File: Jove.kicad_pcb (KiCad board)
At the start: 2 copper layers, 65 x 100 mm, 156 parts, among them J1 PJ301B, J2 PJ301B, J3 PJ301B, J4 PJ301B, J5 PJ301B, J6 PJ301B, P1 CONN_02X05, Q1 BCM857BS, Q2 BCM857BS, Q3 J112, Q4 J112, Q5 J112, Q6 J112, SW1 KS-01Q, U1 TL072-, U10 CD4027, U11 CD40106, U12 TS321, U13 TS321, U2 TL072-, U3 TL072-, U4 TL072-, U5 LM13700, U6 LM13700, U7 LM13700, U8 DG409, U9 CD4052

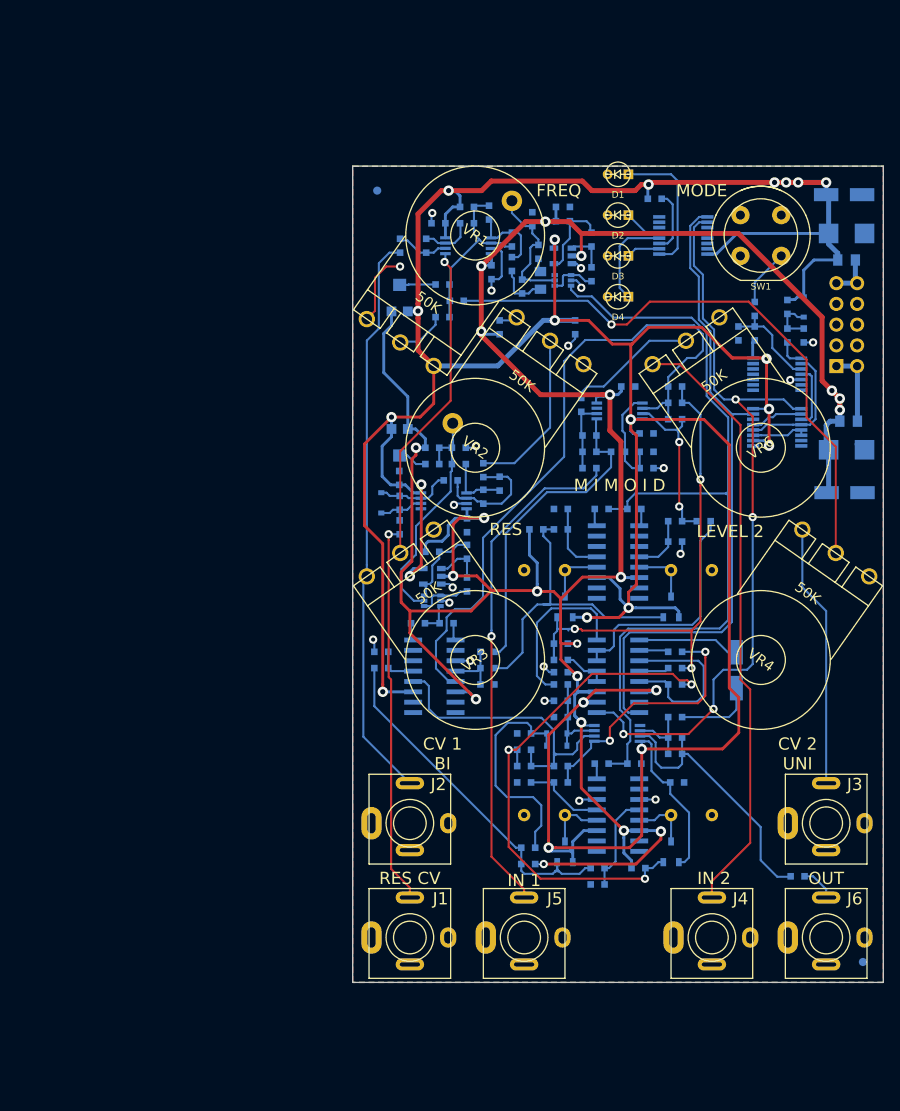
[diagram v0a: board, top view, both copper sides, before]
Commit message: redesign PCB
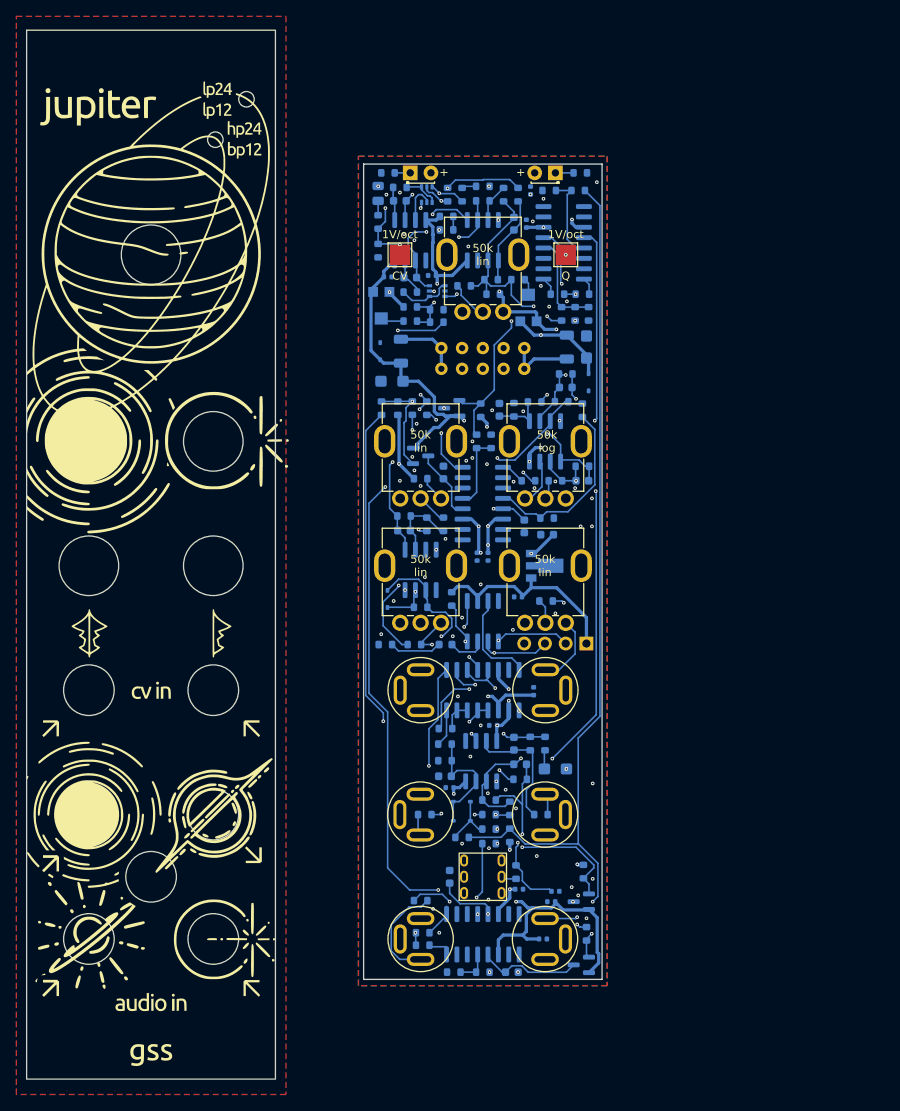
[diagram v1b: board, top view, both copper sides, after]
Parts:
- removed D4: LED, MyModules:3MM-LED-C1A2
- removed D7: 1N914, MyModules:SOD323-C1A2
- removed the REF** at (15.0, 15.0)
- removed the REF** at (74.5, 109.5)
- removed REF***: OSHW-Symbol_6.7x6mm_SilkScreen, Symbols:OSHW-Symbol_6.7x6mm_SilkScreen
- removed U11: CD40106, Housings_SSOP:TSSOP-14_4.4x5mm_Pitch0.65mm
- removed U13: TS321, TO_SOT_Packages_SMD:SOT-23-5
- added C30: 100n, Capacitor_SMD:C_0402_1005Metric, B.Cu at (36.8, 100.8)
- added C31: 100n, Capacitor_SMD:C_0402_1005Metric, B.Cu at (35.3, 106.7)
- added C32: 100n, Capacitor_SMD:C_0402_1005Metric, B.Cu at (32.4, 100.6)
- added G***: LOGO, LOGO, F.Cu at (-10.2, 59.4)
- added G***: LOGO, LOGO, F.Cu at (27.9, 59.4)
- added G***: LOGO, LOGO, F.Cu at (-12.8, 59.5)
- added J7: prog, Connector_PinHeader_2.54mm:PinHeader_1x04_P2.54mm_Vertical, B.Cu at (40.6, 70.5)
- added R79: 470k, Resistor_SMD:R_0603_1608Metric, B.Cu at (23.5, 18.2)
- added R80: 470k, Resistor_SMD:R_0603_1608Metric, B.Cu at (27.9, 14.5)
- added REF**: RK097_Drill_Hole_Panel, Genson_Drill_Holes:RK097_Drill_Hole_Panel, F.Cu at (-20.3, 45.7)
- added REF**: PJ392_Drill_Hole_Panel, Genson_Drill_Holes:PJ392_Drill_Hole_Panel, F.Cu at (-20.3, 76.2)
- added REF**: PJ392_Drill_Hole_Panel, Genson_Drill_Holes:PJ392_Drill_Hole_Panel, F.Cu at (-5.08, 91.4)
- added REF**: PJ392_Drill_Hole_Panel, Genson_Drill_Holes:PJ392_Drill_Hole_Panel, F.Cu at (-20.3, 91.4)
- added REF**: PJ392_Drill_Hole_Panel, Genson_Drill_Holes:PJ392_Drill_Hole_Panel, F.Cu at (-5.08, 76.2)
- added REF**: RK097_Drill_Hole_Panel, Genson_Drill_Holes:RK097_Drill_Hole_Panel, F.Cu at (-20.3, 61.0)
- added REF**: PJ392_Drill_Hole_Panel, Genson_Drill_Holes:PJ392_Drill_Hole_Panel, F.Cu at (-5.08, 106.7)
- added REF**: 6mm_cap_Drill_Hole_Panel, Genson_Drill_Holes:6mm_cap_Drill_Hole_Panel, F.Cu at (-12.7, 99.1)
- added REF**: PJ392_Drill_Hole_Panel, Genson_Drill_Holes:PJ392_Drill_Hole_Panel, F.Cu at (-20.3, 106.7)
- added REF**: LED_1.8mm_Drill_Hole_Panel, Genson_Drill_Holes:LED_1.8mm_Drill_Hole_Panel, F.Cu at (-4.83, 8.76)
- added REF**: RK097_Drill_Hole_Panel, Genson_Drill_Holes:RK097_Drill_Hole_Panel, F.Cu at (-12.7, 22.9)
- added REF**: 6HP_Front_Panel, Genson_Front_Panels:6HP_Front_Panel, F.Cu at (-27.9, -4.65)
- added REF**: RK097_Drill_Hole_Panel, Genson_Drill_Holes:RK097_Drill_Hole_Panel, F.Cu at (-5.08, 45.7)
- added REF**: LED_1.8mm_Drill_Hole_Panel, Genson_Drill_Holes:LED_1.8mm_Drill_Hole_Panel, F.Cu at (-1.02, 3.81)
- added REF**: RK097_Drill_Hole_Panel, Genson_Drill_Holes:RK097_Drill_Hole_Panel, F.Cu at (-5.08, 61.0)
- C1, C11, C2, C28, C29, C3, C4, C5, C8, C9: footprint MyModules:SM0603-C-JRL -> Capacitor_SMD:C_0603_1608Metric
- C10, C23, C24: footprint Capacitors_SMD:c_elec_5x5.3 -> Capacitor_Tantalum_SMD:CP_EIA-3216-18_Kemet-A
- C12, C13, C14, C15, C16, C17, C19, C20, C26, C27: footprint MyModules:SM0603-C-JRL -> Capacitor_SMD:C_0402_1005Metric
- C18, C25, C6, C7: footprint MyModules:CAP-BOX-PFR-5MM -> Capacitor_SMD:C_0603_1608Metric
- C21: value 0.47μ -> 330n; footprint MyModules:SM0603-C-JRL -> Capacitor_SMD:C_0603_1608Metric
- C22: value 0.47μ -> 100n; footprint MyModules:SM0603-C-JRL -> Capacitor_SMD:C_0402_1005Metric
- D1, D2: value LED -> red; footprint MyModules:3MM-LED-C1A2 -> LED_THT:LED_D1.8mm_W3.3mm_H2.4mm
- D10, D5, D6: footprint MyModules:SOD323-C1A2 -> Diode_SMD:D_SOD-323
- D3: value LED -> debug led; footprint MyModules:3MM-LED-C1A2 -> Diode_SMD:D_0603_1608Metric; moved to B.Cu
- D8, D9: value S1BB -> B5819WS; footprint MyModules:SMB-1C2A -> Diode_SMD:D_SOD-323
- J1: value PJ301B -> Resonance CV; footprint MyModules:PJ-301B-JACK-SLOTS -> Genson_Jacks:Jack_3.5mm_PJ392_Vertical
- J2: value PJ301B -> Bipolar Freq CV; footprint MyModules:PJ-301B-JACK-SLOTS -> Genson_Jacks:Jack_3.5mm_PJ392_Vertical
- J3: value PJ301B -> Unipolar Freq CV; footprint MyModules:PJ-301B-JACK-SLOTS -> Genson_Jacks:Jack_3.5mm_PJ392_Vertical
- J4, J5: value PJ301B -> Input2; footprint MyModules:PJ-301B-JACK-SLOTS -> Genson_Jacks:Jack_3.5mm_PJ392_Vertical
- J6: value PJ301B -> out; footprint MyModules:PJ-301B-JACK-SLOTS -> Genson_Jacks:Jack_3.5mm_PJ392_Vertical
- P1: footprint Pin_Headers:Pin_Header_Straight_2x05 -> Genson_Connectors:Eurorack_10Pin
- Q1, Q2: footprint SMD TRAN:sot323-6 -> Package_TO_SOT_SMD:SOT-363_SC-70-6
- Q3, Q4, Q5, Q6: footprint MyModules:SOT23-JRL -> Package_TO_SOT_SMD:SOT-23
- R1, R10, R11, R12, R13, R14, R15, R16, R17, R18, R2, R20, R22, R23, R24, R25, R26, R27, R29, R3, R30, R31, R32, R33, R34, R35, R36, R37, R38, R39, R4, R40, R42, R43, R44, R45, R46, R47, R48, R49, R5, R50, R51, R52, R53, R54, R55, R56, R57, R59, R6, R60, R62, R63, R64, R65, R68, R69, R7, R70, R71, R72, R73, R74, R75, R76, R77, R78, R8, R9: footprint MyModules:SM0603-R-JRL -> Resistor_SMD:R_0603_1608Metric
- R19: footprint MyModules:SM0805-HAND -> Resistor_SMD:R_0805_2012Metric
- R21, R28: value 1.5M -> 1M; footprint MyModules:SM0603-R-JRL -> Resistor_SMD:R_0603_1608Metric
- R41: value 3.3K -> 100k; footprint MyModules:SM0603-R-JRL -> Resistor_SMD:R_0603_1608Metric
- R58: value 33K -> 1k; footprint MyModules:SM0603-R-JRL -> Resistor_SMD:R_0603_1608Metric
- R61: value 100K -> 330; footprint MyModules:SM0603-R-JRL -> Resistor_SMD:R_0603_1608Metric
- R66, R67: footprint MyModules:SM0805-HAND -> Resistor_SMD:R_1206_3216Metric
- SW1: value KS-01Q -> SW_Push_DPDT; footprint synth:KS-01Q-02-JRL -> Genson_Switches:SW_5.8x5.8mm
- TP1, TP2: footprint MyModules:TEST POINT -> TestPoint:TestPoint_Pad_2.5x2.5mm; moved to F.Cu
- U1, U2, U3, U4: footprint MyModules:TSSOP8-JRL -> Package_SO:SOIC-8_3.9x4.9mm_P1.27mm
- U10: value CD4027 -> ~; footprint Housings_SSOP:TSSOP-16_4.4x5mm_Pitch0.65mm -> Package_SO:SOIC-8_3.9x4.9mm_P1.27mm
- U12: value TS321 -> TL072-; footprint TO_SOT_Packages_SMD:SOT-23-5 -> Package_SO:SOIC-8_3.9x4.9mm_P1.27mm
- U5, U6, U7, U8: footprint MyModules:SO16-JRL -> Package_SO:SOIC-16_3.9x9.9mm_P1.27mm
- U9: value CD4052 -> L78L05; footprint Housings_SSOP:TSSOP-16_4.4x5mm_Pitch0.65mm -> Package_TO_SOT_SMD:SOT-89-3
- VR1, VR2, VR3, VR4, VR6: footprint MyModules:RV16A-41-JRL -> Genson_Potentiometers:Potentiometer_RK09_RV09_Vertical
- VR5, VR7: footprint MyModules:TC33X-2 -> Potentiometer_SMD:Potentiometer_Bourns_TC33X_Vertical
- moved SW1 85.6 mm to (27.9, 99.1), turned to 90 degrees
- moved C26 84.2 mm to (36.3, 102.1)
- moved R58 72.2 mm to (32.0, 98.5)
- moved C19 71.4 mm to (16.3, 25.6)
- moved C27 63.3 mm to (23.9, 88.1), turned to 0 degrees
- moved R60 63.3 mm to (39.6, 15.0), turned to 0 degrees
- moved R64 61.1 mm to (16.0, 70.6), turned to 180 degrees
- moved R62 60.1 mm to (36.1, 15.0)
- moved C23 59.9 mm to (16.8, 38.4)
- moved D8 58.9 mm to (15.4, 34.7), turned to 90 degrees
- moved R8 56.9 mm to (20.3, 102.0)
- moved R66 55.7 mm to (17.9, 34.7), turned to 90 degrees
- moved U6 55.4 mm to (37.8, 21.4), turned to 0 degrees
- moved C20 55.1 mm to (33.3, 19.1), turned to -90 degrees
- moved R41 55.0 mm to (24.1, 65.0), turned to -90 degrees
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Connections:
- C2 pad 2: Net-(C2-Pad2) -> Net-(Q1-C1)
- C21 pad 1: Net-(C21-Pad1) -> +12V
- C22 pad 1: Net-(C22-Pad1) -> +5V
- C5 pad 2: Net-(C5-Pad2) -> Net-(Q2-C1)
- D1 pad 1: GND -> Net-(D1-K)
- D1 pad 2: Net-(D1-Pad2) -> /Rx
- D2 pad 1: GND -> Net-(D2-K)
- D2 pad 2: Net-(D2-Pad2) -> /Tx
- D3 pad 1: GND -> Net-(D3-K)
- D3 pad 2: Net-(D3-Pad2) -> Net-(D3-A)
- Q1 pad 6: Net-(C2-Pad2) -> Net-(Q1-C1)
- Q2 pad 6: Net-(C5-Pad2) -> Net-(Q2-C1)
- R21 pad 1: Net-(C2-Pad2) -> Net-(Q1-C1)
- R21 pad 2: -12V -> Net-(R21-Pad2)
- R28 pad 1: Net-(C5-Pad2) -> Net-(Q2-C1)
- R28 pad 2: -12V -> Net-(R28-Pad2)
- R4 pad 2: Net-(J1-Pad3) -> Net-(J1-PadT)
- R41 pad 1: +12V -> +5V
- R41 pad 2: Net-(R41-Pad2) -> Net-(U10-P3.3)
- R54 pad 1: Net-(J6-Pad3) -> Net-(J6-PadT)
- R58 pad 1: Net-(C21-Pad1) -> Net-(U10-P3.3)
- R58 pad 2: +12V -> Net-(R58-Pad2)
- R59 pad 1: Net-(R59-Pad1) -> Net-(D1-K)
- R59 pad 2: Net-(C22-Pad1) -> GND
- R61 pad 1: Net-(C22-Pad1) -> Net-(D2-K)
- R61 pad 2: +12V -> GND
- R64 pad 1: Net-(C21-Pad1) -> Net-(D3-K)
- R64 pad 2: Net-(R64-Pad2) -> GND
- R76 pad 2: Net-(J2-Pad3) -> Net-(J2-PadT)
- R8 pad 2: Net-(J5-Pad3) -> Net-(J5-PadT)
- SW1 pad 1: Net-(R64-Pad2) -> +5V
- SW1 pad 2: GND -> Net-(R58-Pad2)
- SW1 pad 3: (no net) -> GND
- SW1 pad 4: (no net) -> unconnected-(SW1-A-Pad4)
- U10 pad 1: Net-(U10-Pad1) -> Net-(U10-P5.4)
- U10 pad 2: Net-(U10-Pad13) -> +5V
- U10 pad 3: Net-(U10-Pad3) -> Net-(U10-P5.5)
- U10 pad 4: Net-(U10-Pad12) -> GND
- U10 pad 5: +12V -> /Rx
- U10 pad 6: +12V -> /Tx
- U10 pad 7: GND -> Net-(D3-A)
- U10 pad 8: GND -> Net-(U10-P3.3)
- U12 pad 1: Net-(C2-Pad1) -> Net-(C5-Pad1)
- U12 pad 2: -12V -> Net-(Q2-C1)
- U12 pad 4: Net-(C2-Pad2) -> -12V
- U12 pad 5: +12V -> GND
- U5 pad 15: Net-(U5-Pad15) -> unconnected-(U5-Pad15)
- U5 pad 2: Net-(U5-Pad2) -> unconnected-(U5-Pad2)
- U6 pad 15: Net-(U6-Pad15) -> unconnected-(U6-Pad15)
- U6 pad 2: Net-(U6-Pad2) -> unconnected-(U6-Pad2)
- U7 pad 15: Net-(U7-Pad15) -> unconnected-(U7-Pad15)
- U7 pad 2: Net-(U7-Pad2) -> unconnected-(U7-Pad2)
- U8 pad 1: Net-(U10-Pad1) -> Net-(U10-P5.4)
- U8 pad 16: Net-(U10-Pad15) -> Net-(U10-P5.5)
- U9 pad 1: Net-(D1-Pad2) -> +5V
- U9 pad 2: Net-(D3-Pad2) -> GND
- U9 pad 3: Net-(R41-Pad2) -> +12V
- VR3 pad 3: Net-(J2-Pad3) -> Net-(J2-PadT)
- VR4 pad 3: Net-(J3-Pad3) -> Net-(J3-PadT)
- VR6 pad 3: Net-(J4-Pad3) -> Net-(J4-PadT)
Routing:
- net +12V: track 500.1 -> 222.5 mm, vias 23 -> 19
- net -12V: track 340.1 -> 216.3 mm, vias 20 -> 22
- net Net-(U10-Pad1): track 94.4 -> 0.00 mm, vias 4 -> 0
- net Net-(U10-Pad15): track 81.0 -> 0.00 mm
- net /Rx: track 0.00 -> 79.0 mm, vias 0 -> 2
- net /Tx: track 0.00 -> 75.5 mm, vias 0 -> 3
- net Net-(J4-Pad3): track 74.2 -> 0.00 mm
- net Net-(U3A--): track 8.96 -> 82.2 mm, vias 0 -> 5
- net Net-(J2-Pad3): track 70.0 -> 0.00 mm
- net Net-(R3-Pad2): track 72.5 -> 2.98 mm, vias 1 -> 0
- net Net-(Q5-S): track 44.3 -> 112.2 mm, vias 0 -> 2
- net +5V: track 0.00 -> 65.3 mm, vias 0 -> 1
- net Net-(J5-Pad3): track 62.4 -> 0.00 mm, vias 1 -> 0
- net Net-(U1B--): track 6.48 -> 67.0 mm, vias 0 -> 3
- net Net-(J4-PadT): track 0.00 -> 60.3 mm, vias 0 -> 2
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- added copper zone on F.Cu, net (none)
- added copper zone on In1.Cu, net GND
- added copper zone on In2.Cu, net GND
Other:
- board size 65 x 100 mm -> 30.5 x 128.5 mm
- copper layers 2 -> 4
- net class Default removed
- net class POWER removed
- board text added: "+"
- board text added: "1V/oct"
- board text added: "50k lin"
- board text added: "50k log"
- board text added: "CV"
- board text added: "Q"
- board text removed: "-12V"
- board text removed: "CV 1 BI"
- board text removed: "CV 2 UNI"
- board text removed: "FREQ"
- board text removed: "FREQ ADJ"
- board text removed: "IN 1"
- board text removed: "IN 2"
- board text removed: "JOVE"
- board text removed: "LEVEL 2"
- board text removed: "M I M O I D"
- board text removed: "MODE"
- board text removed: "Multimode Filter v1.4 01 2017"
- board text removed: "OUT"
- board text removed: "RES"
- board text removed: "RES ADJ"
- board text removed: "RES CV"
- board text removed: "system80.net"
